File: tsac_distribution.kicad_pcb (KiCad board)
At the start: 2 copper layers, 92 x 82 mm, 45 parts, among them J1 Conn_01x23, J2 Conn_01x02, J21 Conn_01x02, J22 Conn_01x02, J23 Conn_01x02, J31 Conn_01x08, J32 Conn_01x02, J33 Conn_01x02, J41 Conn_01x02, J42 Conn_01x02, J43 Conn_01x02, J44 Conn_01x02, J45 Conn_01x08, J51 Conn_01x03, J61 Conn_01x02, J62 Conn_01x02

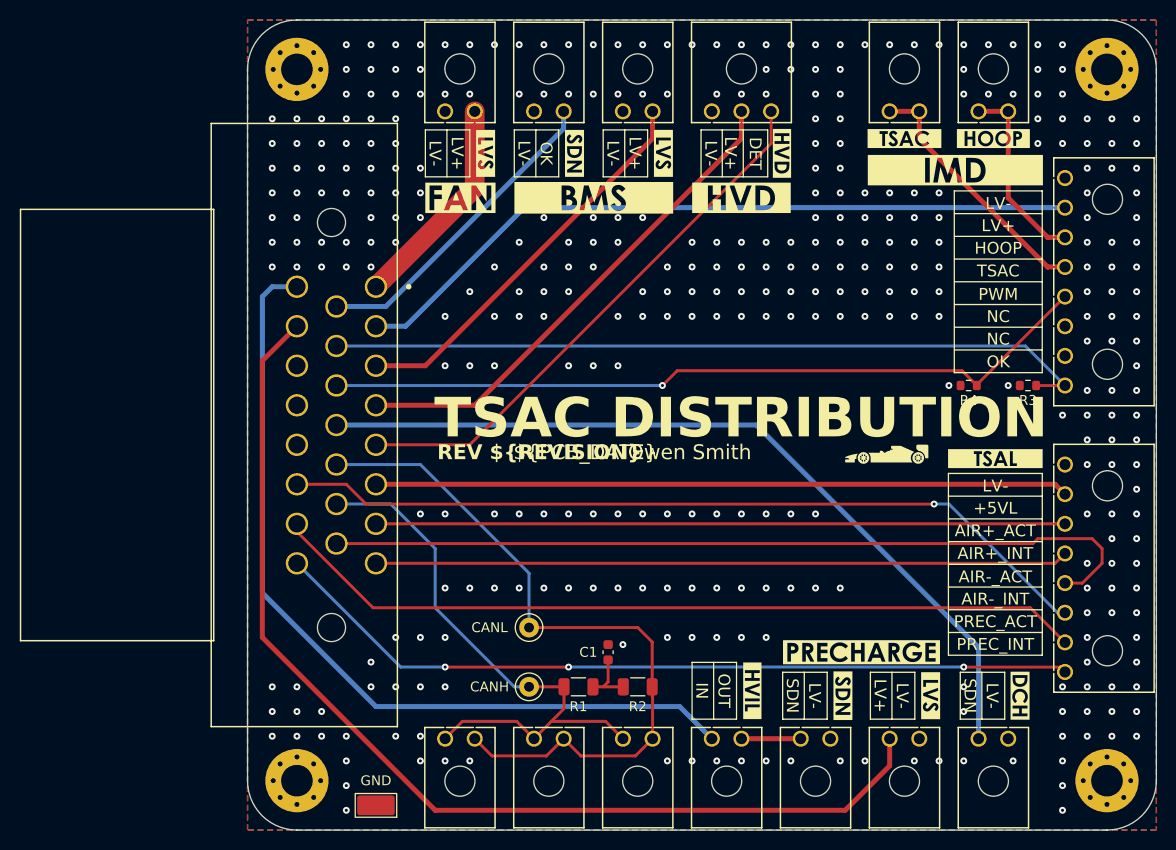
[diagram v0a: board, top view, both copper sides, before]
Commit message: pcb: Run track cleanup
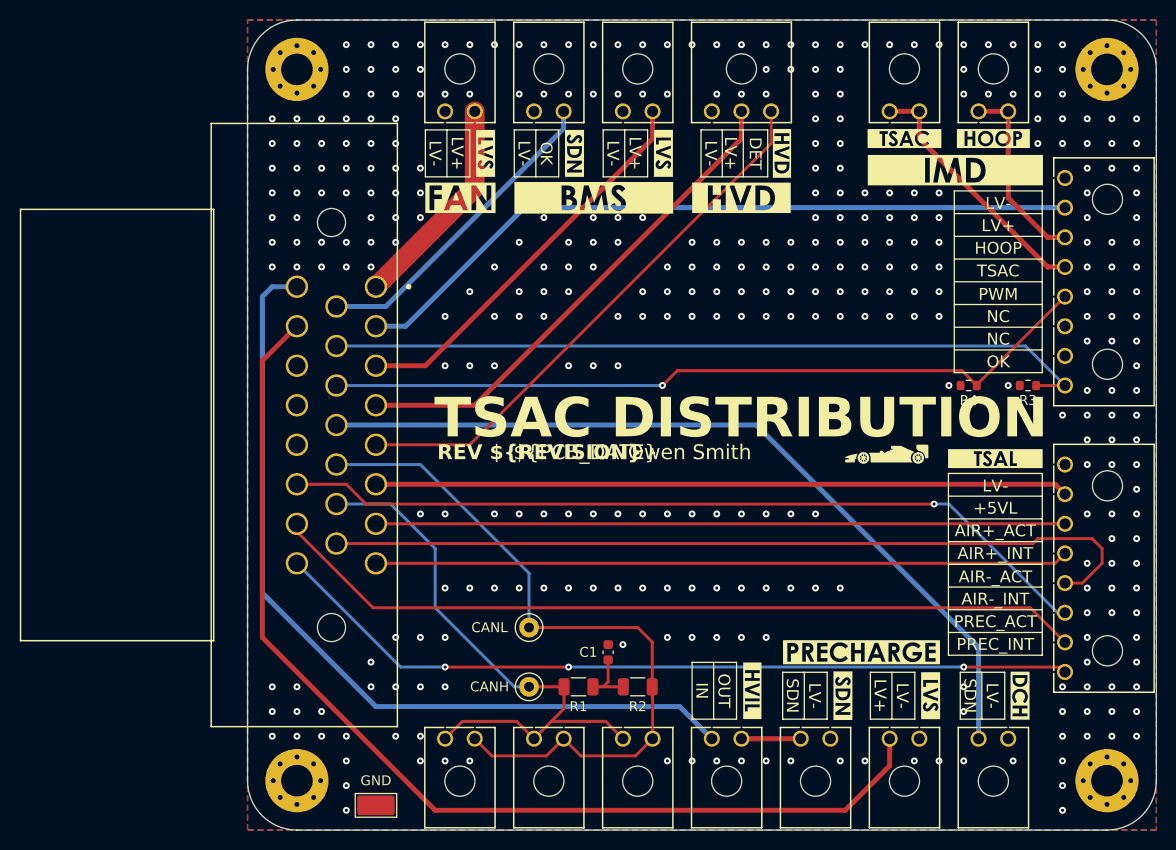
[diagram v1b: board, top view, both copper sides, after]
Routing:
- net PRCHG_ACT: track 83.2 -> 82.4 mm
- net PRCHG_INT: track 83.0 -> 82.3 mm
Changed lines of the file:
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@@
 				(font
 					(size 0.001 0.001)
+					(thickness 0.15)
 				)
 			)
@@
 				(font
 					(size 0.001 0.001)
+					(thickness 0.15)
 				)
 			)
@@
 				(font
 					(size 0.001 0.001)
+					(thickness 0.15)
 				)
 			)
@@
 				(font
 					(size 0.001 0.001)
+					(thickness 0.15)
 				)
 			)
@@
 				(font
 					(size 0.001 0.001)
+					(thickness 0.15)
 				)
 			)
@@
 				(font
 					(size 0.001 0.001)
+					(thickness 0.15)
 				)
 			)
@@
 				(font
 					(size 0.001 0.001)
+					(thickness 0.15)
 				)
 			)
@@
 				(font
 					(size 0.001 0.001)
+					(thickness 0.15)
 				)
 			)
@@
 				(font
 					(size 0.001 0.001)
+					(thickness 0.15)
 				)
 			)
@@
 				(font
 					(size 0.001 0.001)
+					(thickness 0.15)
 				)
 			)
@@
 				(font
 					(size 0.001 0.001)
+					(thickness 0.15)
 				)
 			)
@@
 				(font
 					(size 0.001 0.001)
+					(thickness 0.15)
 				)
 			)
@@
 				(font
 					(size 0.001 0.001)
+					(thickness 0.15)
 				)
 			)
@@
 				(font
 					(size 0.001 0.001)
+					(thickness 0.15)
 				)
 			)
@@
 				(font
 					(size 0.001 0.001)
+					(thickness 0.15)
 				)
 			)
@@
 				(font
 					(size 0.001 0.001)
+					(thickness 0.15)
 				)
 			)
@@
 	)
 	(segment
-		(start 162.250006 105.5)
-		(end 162.75 105.999994)
-		(width 0.3)
-		(layer "B.Cu")
-		(net 4)
-	)
-	(segment
 		(start 110.750001 111)
 		(end 116.250001 111)
@@
 	)
 	(segment
-		(start 85 91.796729)
-		(end 85 90.999998)
-		(width 0.3)
-		(layer "F.Cu")
-		(net 7)
-	)
-	(segment
 		(start 131.499998 80.999998)
 		(end 154 103.5)
@@
 	)
 	(segment
-		(start 89 92.999997)
-		(end 89.000003 93)
-		(width 0.3)
-		(layer "F.Cu")
-		(net 13)
-	)
-	(segment
 		(start 89.000003 93)
 		(end 159.5 93)
@@
 	)
 	(segment
-		(start 159.825006 76.999994)
-		(end 159.825 77)
-		(width 0.3)
-		(layer "F.Cu")
-		(net 14)
-	)
-	(segment
 		(start 158.750005 72.999999)
 		(end 162.75 76.999994)
@@
 	)
 	(segment
-		(start 160.5 59)
-		(end 108 59)
-		(width 0.5)
-		(layer "B.Cu")
-		(net 15)
-	)
-	(segment
-		(start 162.75 58.999999)
-		(end 160.5 59)
+		(start 108 59)
+		(end 162.75 58.999999)
 		(width 0.5)
 		(layer "B.Cu")
@@
 	)
 	(segment
-		(start 153.825 77)
-		(end 153.825 76.924997)
-		(width 0.3)
-		(layer "F.Cu")
-		(net 17)
-	)
-	(segment
 		(start 123.5 75.5)
 		(end 122 77)
@@
 		(width 0.3)
 		(layer "F.Cu")
-		(net 17)
-	)
-	(segment
-		(start 162.749997 68)
-		(end 162.75 67.999997)
-		(width 0.3)
-		(layer "F.Cu")
